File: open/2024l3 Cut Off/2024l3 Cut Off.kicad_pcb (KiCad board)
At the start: 2 copper layers, 174 x 119 mm, 22 parts, among them J1 Conn_01x06, J2 TOF 0, J3 TOF 1, J4 TOF 2, J5 TOF 3, U1 OpenMV, U2 4754, U3 xiao-esp32c3, U4 Adafruit Featherwing, U5 Teensy 4.0

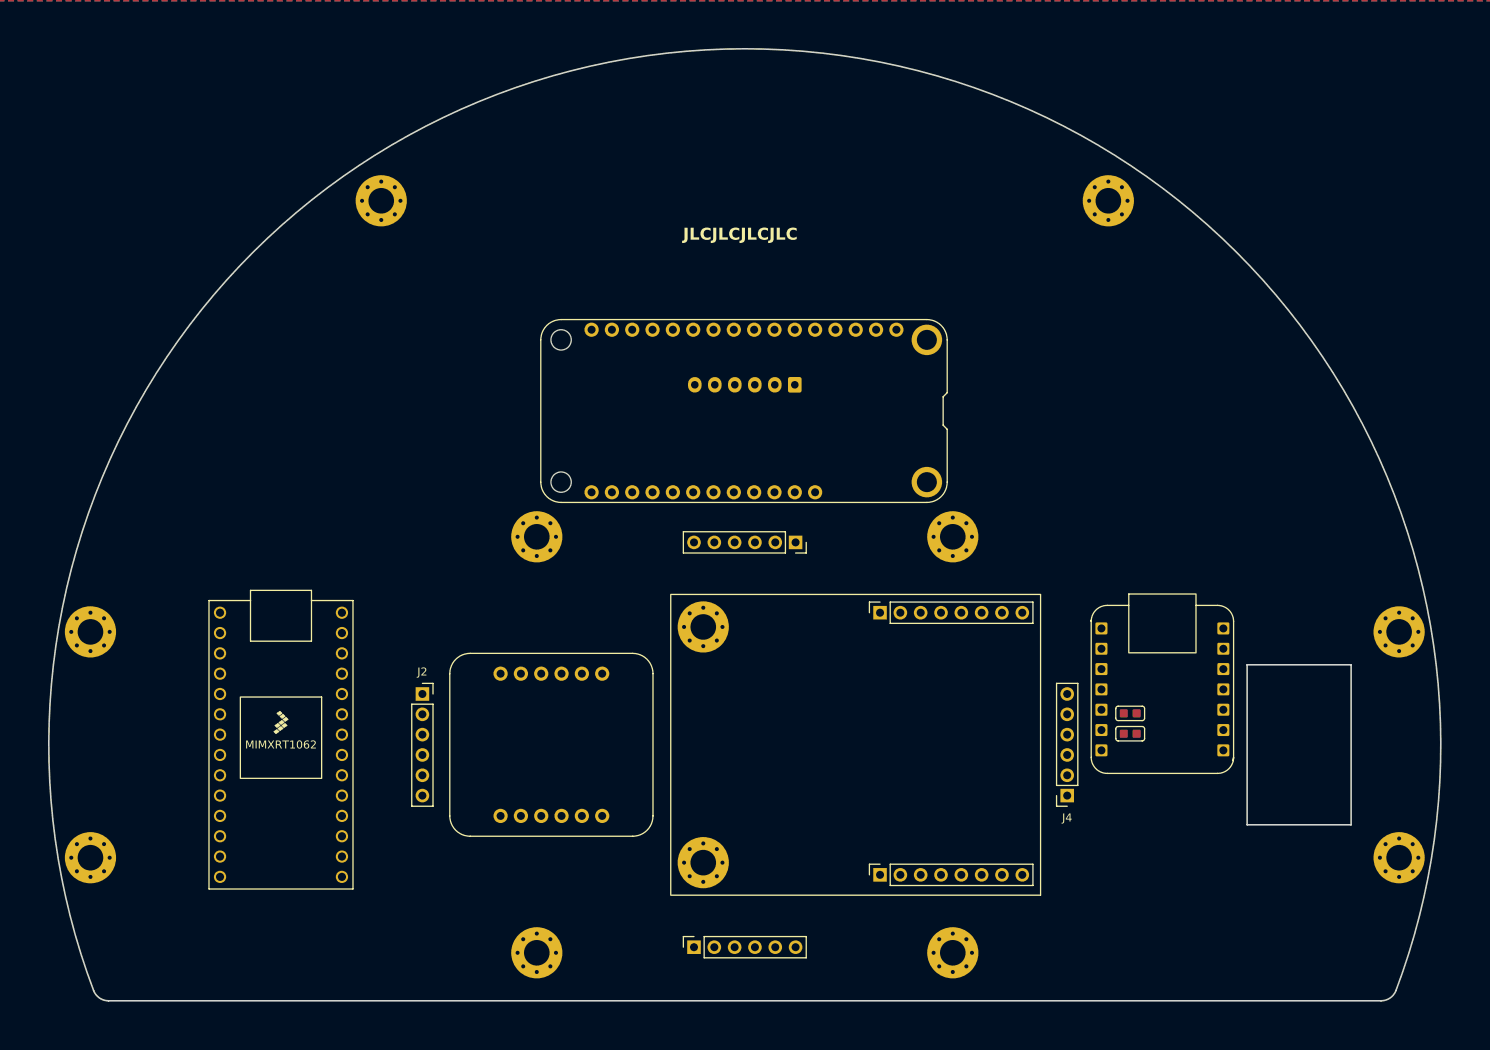
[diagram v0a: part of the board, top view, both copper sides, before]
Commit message: STEP FIle
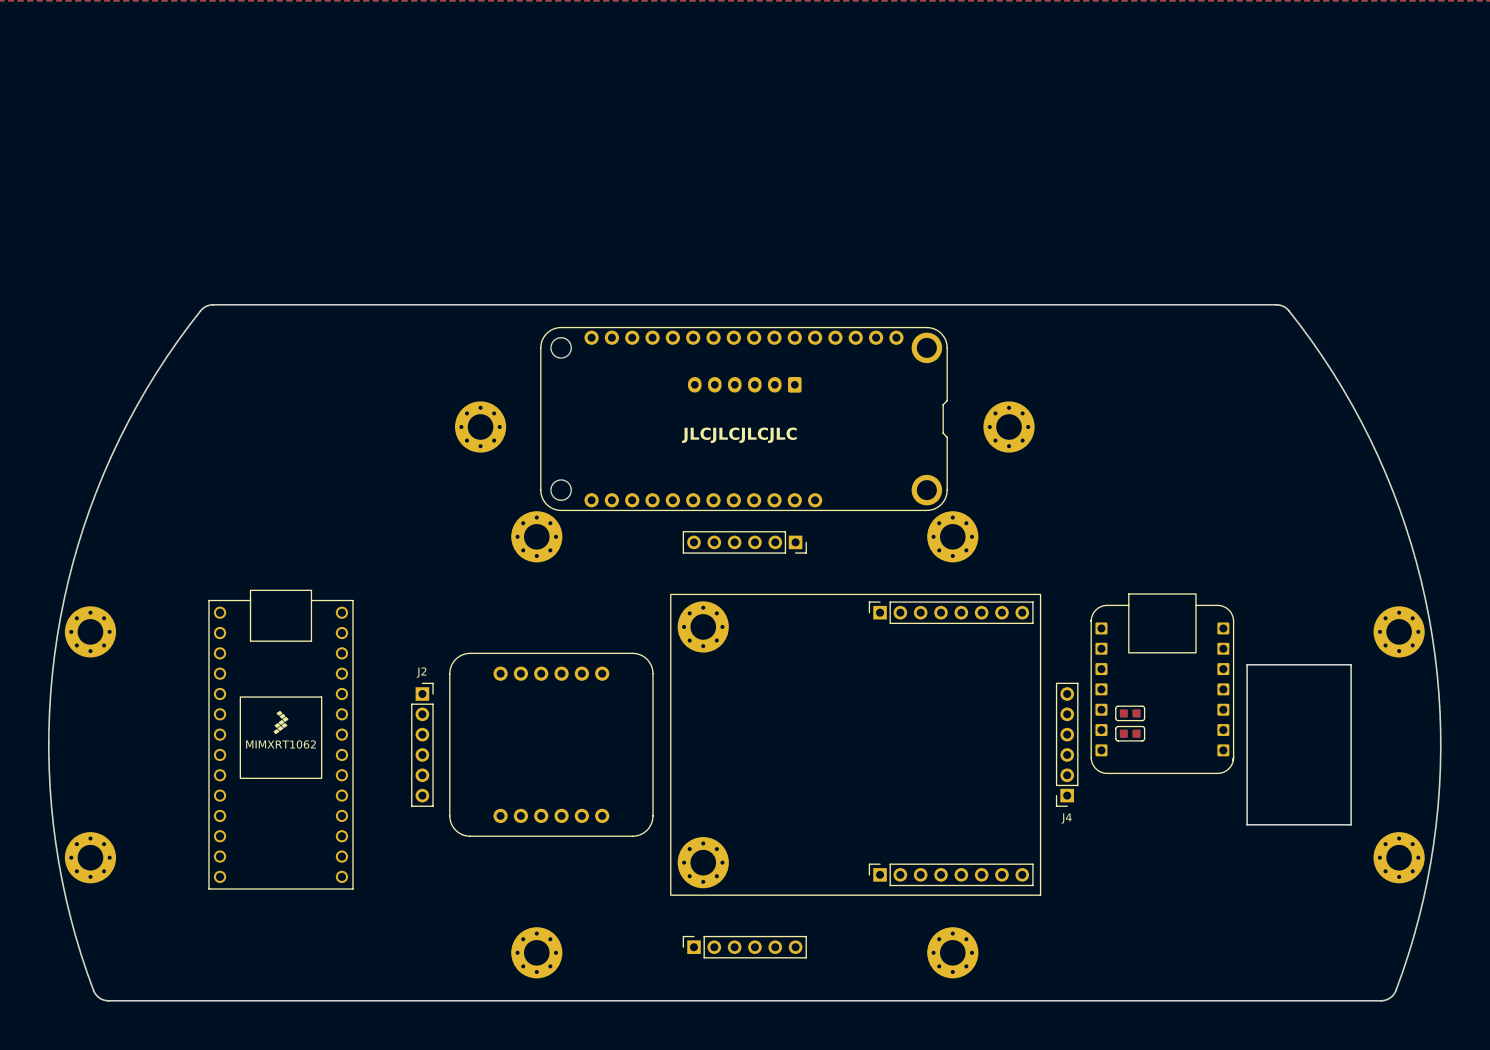
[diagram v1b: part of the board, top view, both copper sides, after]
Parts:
- moved H7 30.9 mm to (181.5, 65.3)
- moved H8 30.9 mm to (115.5, 65.3)
- moved U4 1.00 mm to (148.5, 64.2)
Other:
- board size 174 x 119 mm -> 174 x 87 mm
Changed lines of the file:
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@@
   )
   (footprint "MountingHole:MountingHole_3.2mm_M3_Pad_Via" (layer "F.Cu")
-    (at 103.052395 37.002422)
+    (at 115.466792 65.278635)
     (descr "Mounting Hole 3.2mm, M3")
     (tags "mounting hole 3.2mm m3")
@@
   )
   (footprint "MountingHole:MountingHole_3.2mm_M3_Pad_Via" (layer "F.Cu")
-    (at 193.939606 37.002422)
+    (at 181.525205 65.278635)
     (descr "Mounting Hole 3.2mm, M3")
     (tags "mounting hole 3.2mm m3")
@@
   )
   (footprint "2024l3:Adafruit Feather OLED" (layer "F.Cu")
-    (at 148.496 63.179 180)
+    (at 148.496 64.179 180)
     (property "Sheetfile" "2024l3 Cut Off.kicad_sch")
     (property "Sheetname" "")
@@
     )
   )
-  (gr_line (start 211.287143 115.004002) (end 211.287143 95.004003)
-    (stroke (width 0.2) (type solid)) (layer "Edge.Cuts"))
-  (gr_arc (start 67.09484 135.709884) (mid 148.496 18.003999) (end 229.897159 135.709884)
-    (stroke (width 0.2) (type solid)) (layer "Edge.Cuts"))
-  (gr_line (start 211.287143 95.004003) (end 224.287143 95.004003)
-    (stroke (width 0.2) (type solid)) (layer "Edge.Cuts"))
-  (gr_line (start 224.287143 115.004002) (end 211.287143 115.004002)
-    (stroke (width 0.2) (type solid)) (layer "Edge.Cuts"))
-  (gr_line (start 68.966131 137.004003) (end 228.025869 137.004003)
-    (stroke (width 0.2) (type solid)) (layer "Edge.Cuts"))
-  (gr_arc (start 68.966131 137.004003) (mid 67.828523 136.648972) (end 67.09484 135.709884)
-    (stroke (width 0.2) (type solid)) (layer "Edge.Cuts"))
-  (gr_line (start 224.287143 95.004003) (end 224.287143 115.004002)
-    (stroke (width 0.2) (type solid)) (layer "Edge.Cuts"))
-  (gr_arc (start 229.897159 135.709884) (mid 229.163462 136.648958) (end 228.025869 137.004003)
-    (stroke (width 0.2) (type solid)) (layer "Edge.Cuts"))
-  (gr_text "JLCJLCJLCJLC" (at 140.771 42.054) (layer "F.SilkS")
+  (gr_arc (start 67.094838 135.709882) (mid 62.556097 91.463932) (end 80.479408 50.75694)
+    (stroke (width 0.2) (type solid)) (layer "Edge.Cuts"))
+  (gr_arc (start 68.966129 137.004) (mid 67.828523 136.648968) (end 67.094838 135.709882)
+    (stroke (width 0.2) (type solid)) (layer "Edge.Cuts"))
+  (gr_arc (start 80.479408 50.75694) (mid 81.175286 50.202043) (end 82.043007 50.004)
+    (stroke (width 0.2) (type solid)) (layer "Edge.Cuts"))
+  (gr_line (start 224.287142 95.003999) (end 224.287142 115.004)
+    (stroke (width 0.2) (type solid)) (layer "Edge.Cuts"))
+  (gr_line (start 214.94899 50.004) (end 82.043007 50.004)
+    (stroke (width 0.2) (type solid)) (layer "Edge.Cuts"))
+  (gr_arc (start 229.897159 135.709882) (mid 229.163461 136.648956) (end 228.025868 137.004)
+    (stroke (width 0.2) (type solid)) (layer "Edge.Cuts"))
+  (gr_line (start 211.287142 115.004) (end 211.287142 95.003999)
+    (stroke (width 0.2) (type solid)) (layer "Edge.Cuts"))
+  (gr_line (start 211.287142 95.003999) (end 224.287142 95.003999)
+    (stroke (width 0.2) (type solid)) (layer "Edge.Cuts"))
+  (gr_line (start 68.966129 137.004) (end 228.025868 137.004)
+    (stroke (width 0.2) (type solid)) (layer "Edge.Cuts"))
+  (gr_arc (start 214.94899 50.004) (mid 215.816711 50.20204) (end 216.512589 50.75694)
+    (stroke (width 0.2) (type solid)) (layer "Edge.Cuts"))
+  (gr_line (start 224.287142 115.004) (end 211.287142 115.004)
+    (stroke (width 0.2) (type solid)) (layer "Edge.Cuts"))
+  (gr_arc (start 216.512589 50.75694) (mid 234.4359 91.463932) (end 229.897159 135.709882)
+    (stroke (width 0.2) (type solid)) (layer "Edge.Cuts"))
+  (gr_text "JLCJLCJLCJLC" (at 140.771 67.054) (layer "F.SilkS")
     (effects (font (size 1.5 1.5) (thickness 0.3) bold) (justify left bottom))
   )
@@
     )
   )
-  (group "" (id d5c53182-f4eb-4ee6-a37b-190a7e240ec7)
+  (group "" (id 187da8aa-159e-4375-a764-e9f66b501069)
     (members
-      0ec7b0be-fae6-4b1a-86a2-e70fa4a870fb
-      108433e7-5be6-430a-a8fe-c9687ab93f13
-      3fbd9048-8f66-4564-b464-fc04d807d5b8
-      4a403a17-aa3c-45cd-bd99-dfb66b715e04
-      5595356c-226e-4fae-ae46-ec121ea8306f
-      c063c772-a7d5-46ff-9b80-64e274719699
-      c4b7e0c8-40b9-4c58-98a0-e147af8b5097
-      cb11e9ae-ab34-42b0-8c97-c229fd758920
-    )
-  )
+      21106090-f5e7-49d6-bdb2-1c002f9a16e3
+      47df7ce1-4407-45b8-a698-bbba8da43787
+      57bdda2a-994b-4006-855e-76fd6243d497
+      5a2a70b5-4362-440d-96fa-72615f4c3de4
+      63bd1780-7daa-4e55-8e3d-3a7c572145e7
+      6464e2b7-11b8-4145-af13-8eed389b98da
+      7127d337-6364-40a2-a53e-5e8c678f1f10
+      730340cb-0144-4975-b9f4-1821ff8194c4
+      7896ad17-8745-4ab9-b3c3-73ffb36cedbb
+      81acd5bf-bab6-4e4c-883e-61ed4dca0122
+      bc86eca1-215c-442b-b8b0-712fb2bdbb35
+      cef757ee-bf34-4741-b341-c479a45f9a03
+    )
+  )
